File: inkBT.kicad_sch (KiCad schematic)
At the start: 10 parts, among them J1 AudioJack2_Ground, U1 LM2596S-3.3, U2 ESP32-WROOM-32, U3 PCM5102A

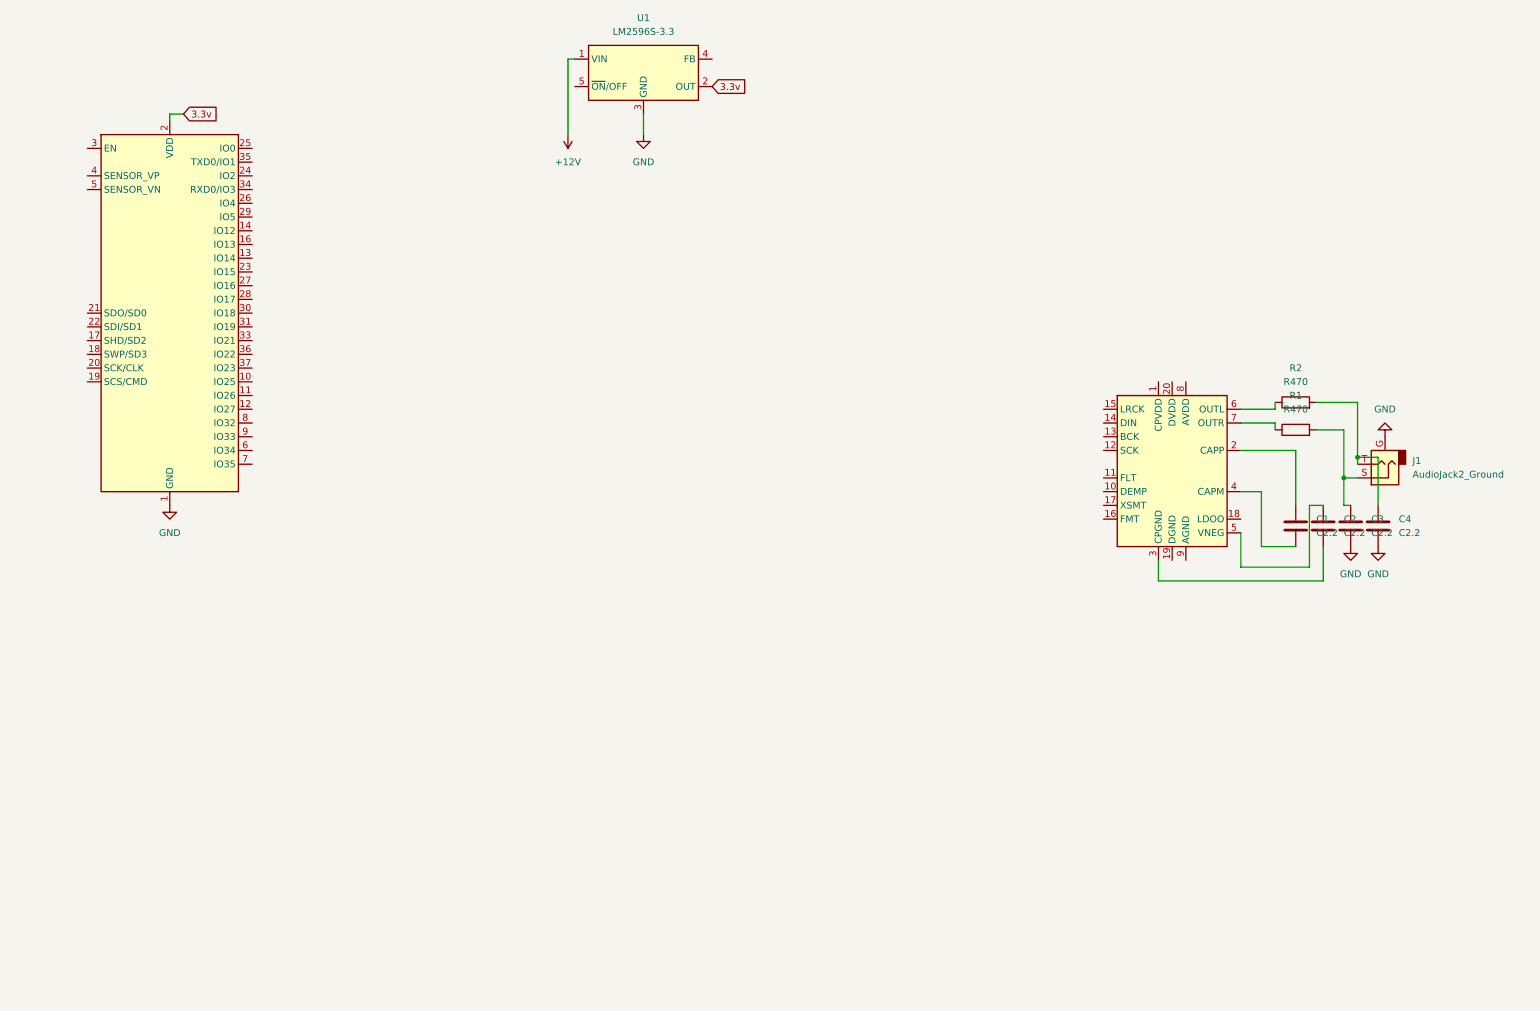
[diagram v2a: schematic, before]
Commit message: a
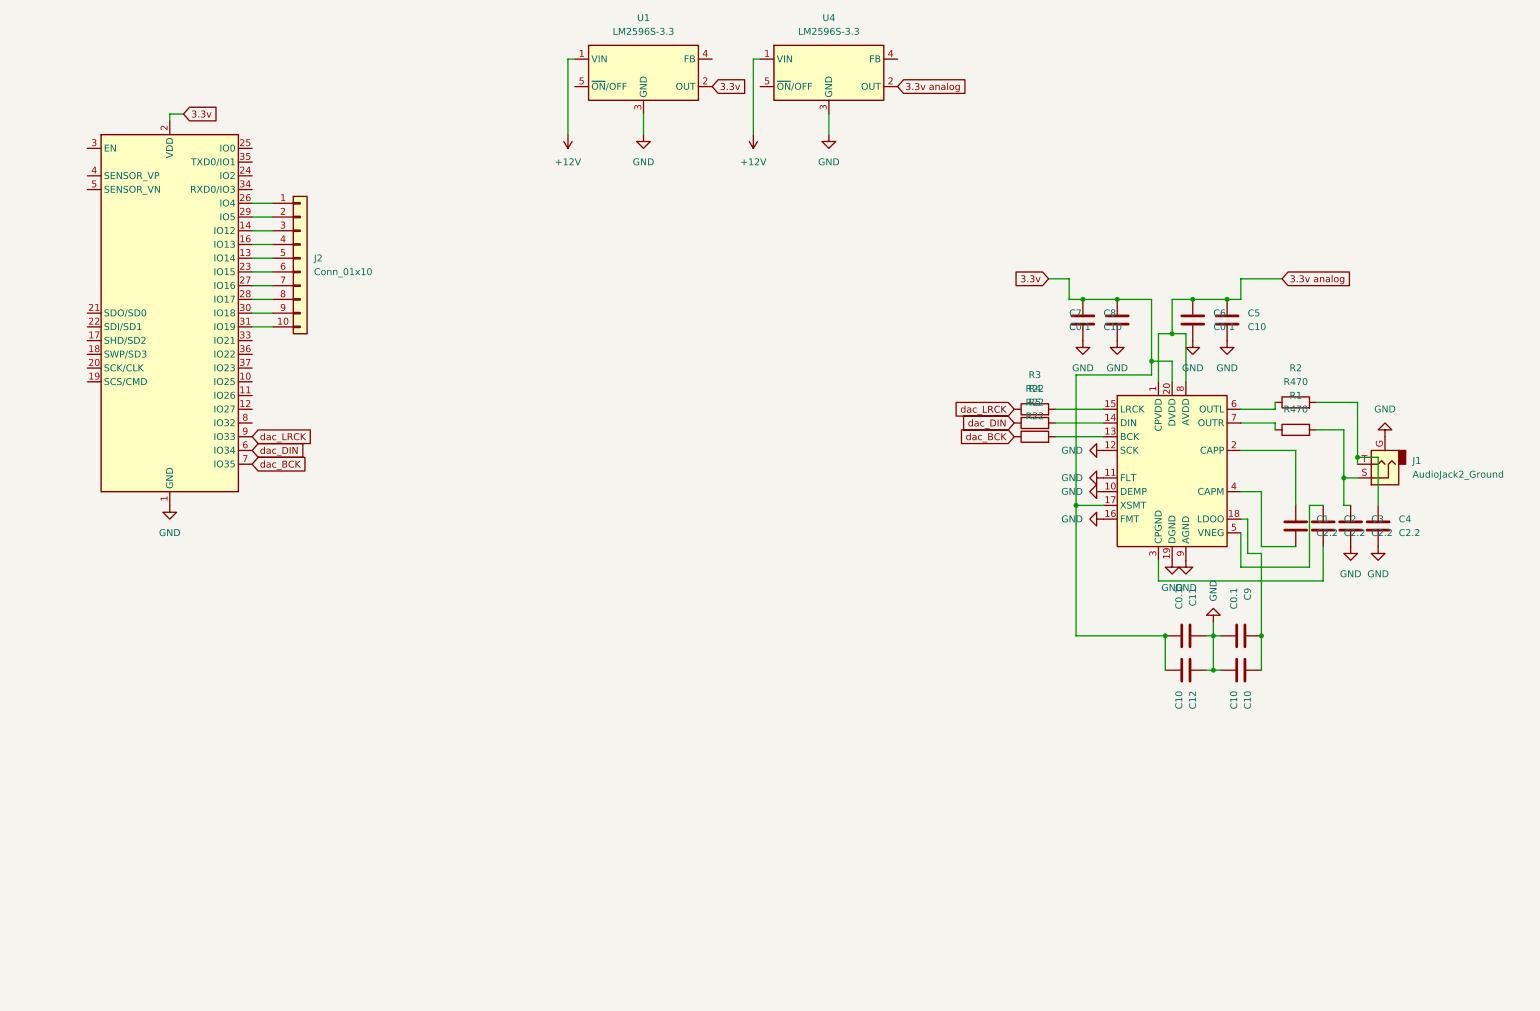
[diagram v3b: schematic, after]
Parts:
- added C10, C12, C5, C8: C10, Capacitor_SMD:C_1206_3216Metric_Pad1.33x1.80mm_HandSolder, symbol Device:C
- added C11, C6, C7, C9: C0.1, Capacitor_SMD:C_1206_3216Metric_Pad1.33x1.80mm_HandSolder, symbol Device:C
- added J2: Conn_01x10, symbol Connector_Generic:Conn_01x10
- added R3, R4, R5: R22, Resistor_SMD:R_1206_3216Metric_Pad1.30x1.75mm_HandSolder, symbol Device:R
- added U4: LM2596S-3.3, Package_TO_SOT_SMD:TO-263-5_TabPin3, symbol Regulator_Switching:LM2596S-3.3
- C1, C2, C3, C4: footprint Package_SO:SOIC-8_3.9x4.9mm_P1.27mm -> Capacitor_SMD:C_1206_3216Metric_Pad1.33x1.80mm_HandSolder
- J1: footprint Connector_Audio:Jack_3.5mm_QingPu_WQP-PJ398SM_Vertical_CircularHoles -> Connector_PinSocket_1.00mm:PinSocket_1x03_P1.00mm_Vertical
- R1, R2: footprint (none) -> Resistor_SMD:R_1206_3216Metric_Pad1.30x1.75mm_HandSolder
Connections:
- net +12V: now also U4.1 (VIN)
- net 3.3v: now also U3.17 (XSMT), U3.20 (DVDD), C11.2, C12.2, C7.1, C8.1
- net GND: now also U3.10 (DEMP), U3.11 (FLT), U3.12 (SCK), U3.16 (FMT), U3.19 (DGND), U3.9 (AGND), C10.2, C11.1, C12.1, C5.2, C6.2, C7.2, C8.2, C9.2, U4.3 (GND)
- net 3.3v analog: now reaches U3.1 (CPVDD)
- net 3.3v analog: now also U3.8 (AVDD), C5.1, C6.1, U4.2 (OUT)
- net at U3.13 (BCK): now also R5.2
- net at U3.14 (DIN): now also R4.2
- net at U3.15 (LRCK): now also R3.2
- net at U3.18 (LDOO): now also C10.1, C9.1
- net at U2.13 (IO14): now also J2.5 (Pin_5)
- net at U2.14 (IO12): now also J2.3 (Pin_3)
- net at U2.16 (IO13): now also J2.4 (Pin_4)
- net at U2.23 (IO15): now also J2.6 (Pin_6)
- net at U2.26 (IO4): now also J2.1 (Pin_1)
- net at U2.27 (IO16): now also J2.7 (Pin_7)
- net at U2.28 (IO17): now also J2.8 (Pin_8)
- net at U2.29 (IO5): now also J2.2 (Pin_2)
- net at U2.30 (IO18): now also J2.9 (Pin_9)
- net at U2.31 (IO19): now also J2.10 (Pin_10)
- net dac_DIN: now reaches U2.6 (IO34)
- net dac_DIN: now also R4.1
- net dac_BCK: now reaches U2.7 (IO35)
- net dac_BCK: now also R5.1
- net dac_LRCK: now reaches U2.9 (IO33)
- net dac_LRCK: now also R3.1

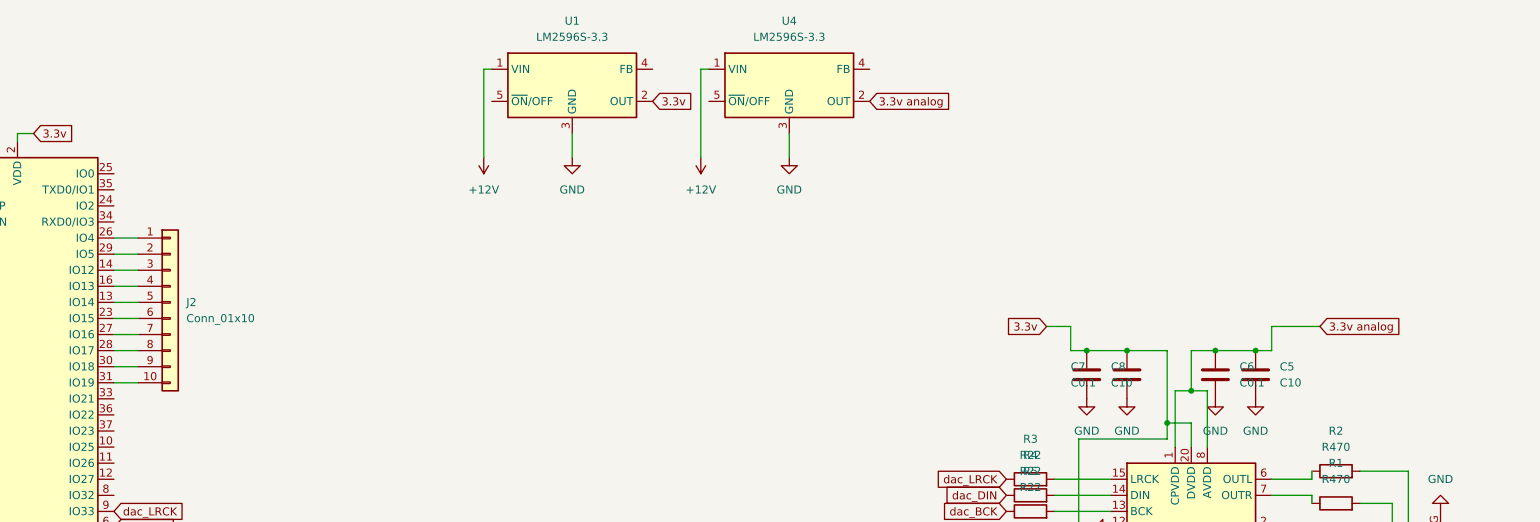
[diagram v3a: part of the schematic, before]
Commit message: a
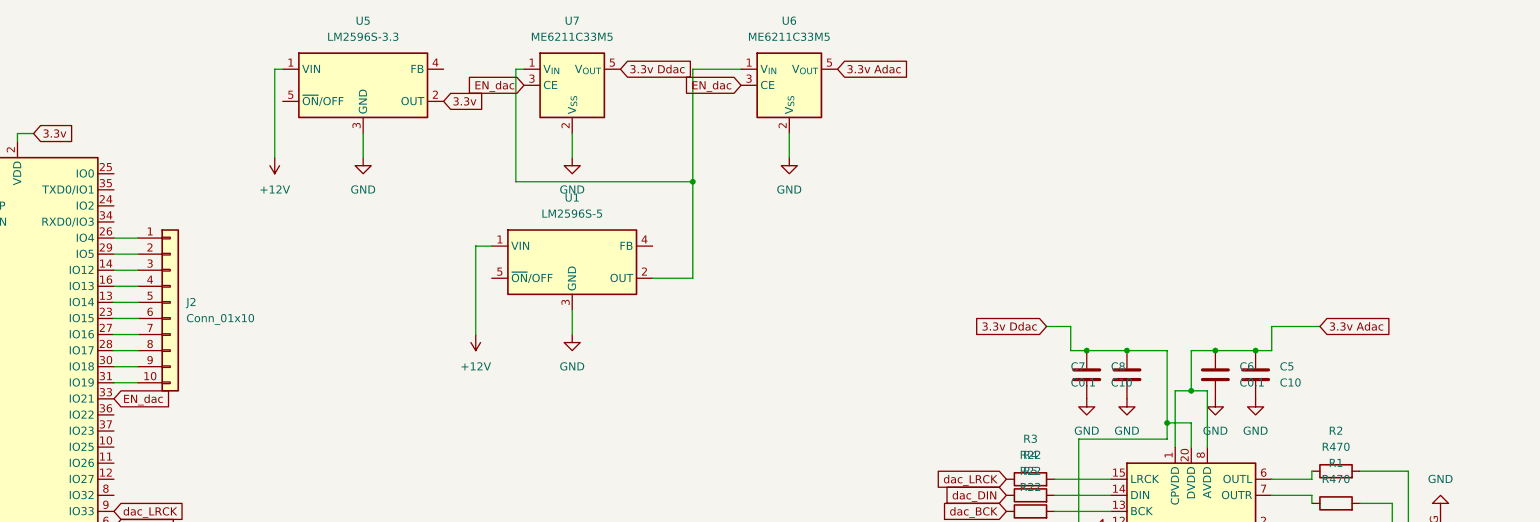
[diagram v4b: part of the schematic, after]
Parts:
- removed U1, U4: LM2596S-3.3, Package_TO_SOT_SMD:TO-263-5_TabPin3, symbol Regulator_Switching:LM2596S-3.3
- added U1: LM2596S-5, Package_TO_SOT_SMD:TO-263-5_TabPin3, symbol Regulator_Switching:LM2596S-5
- added U5: LM2596S-3.3, Package_TO_SOT_SMD:TO-263-5_TabPin3, symbol Regulator_Switching:LM2596S-3.3
- added U6, U7: ME6211C33M5, Package_TO_SOT_SMD:SOT-23-5, symbol Regulator_Linear:ME6211C33M5
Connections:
- net +12V: now also U1.1 (VIN), U5.1 (VIN)
- net 3.3v: now also U5.2 (OUT); no longer C11.2, C12.2, C7.1, C8.1, U3.17 (XSMT), U3.20 (DVDD)
- net GND: now also U1.3 (GND), U5.3 (GND), U6.2 (V_{SS}), U7.2 (V_{SS})
- net EN_dac: now reaches U2.33 (IO21)
- net EN_dac: now also U6.3 (CE), U7.3 (CE)
- net 3.3v analog renamed 3.3v Adac
- net 3.3v Adac: now also U6.5 (V_{OUT})
- new net: U1.2 (OUT), U6.1 (V_{IN}), U7.1 (V_{IN})
- new net 3.3v Ddac: C11.2, C12.2, C7.1, C8.1, U3.17 (XSMT), U3.20 (DVDD), U7.5 (V_{OUT})

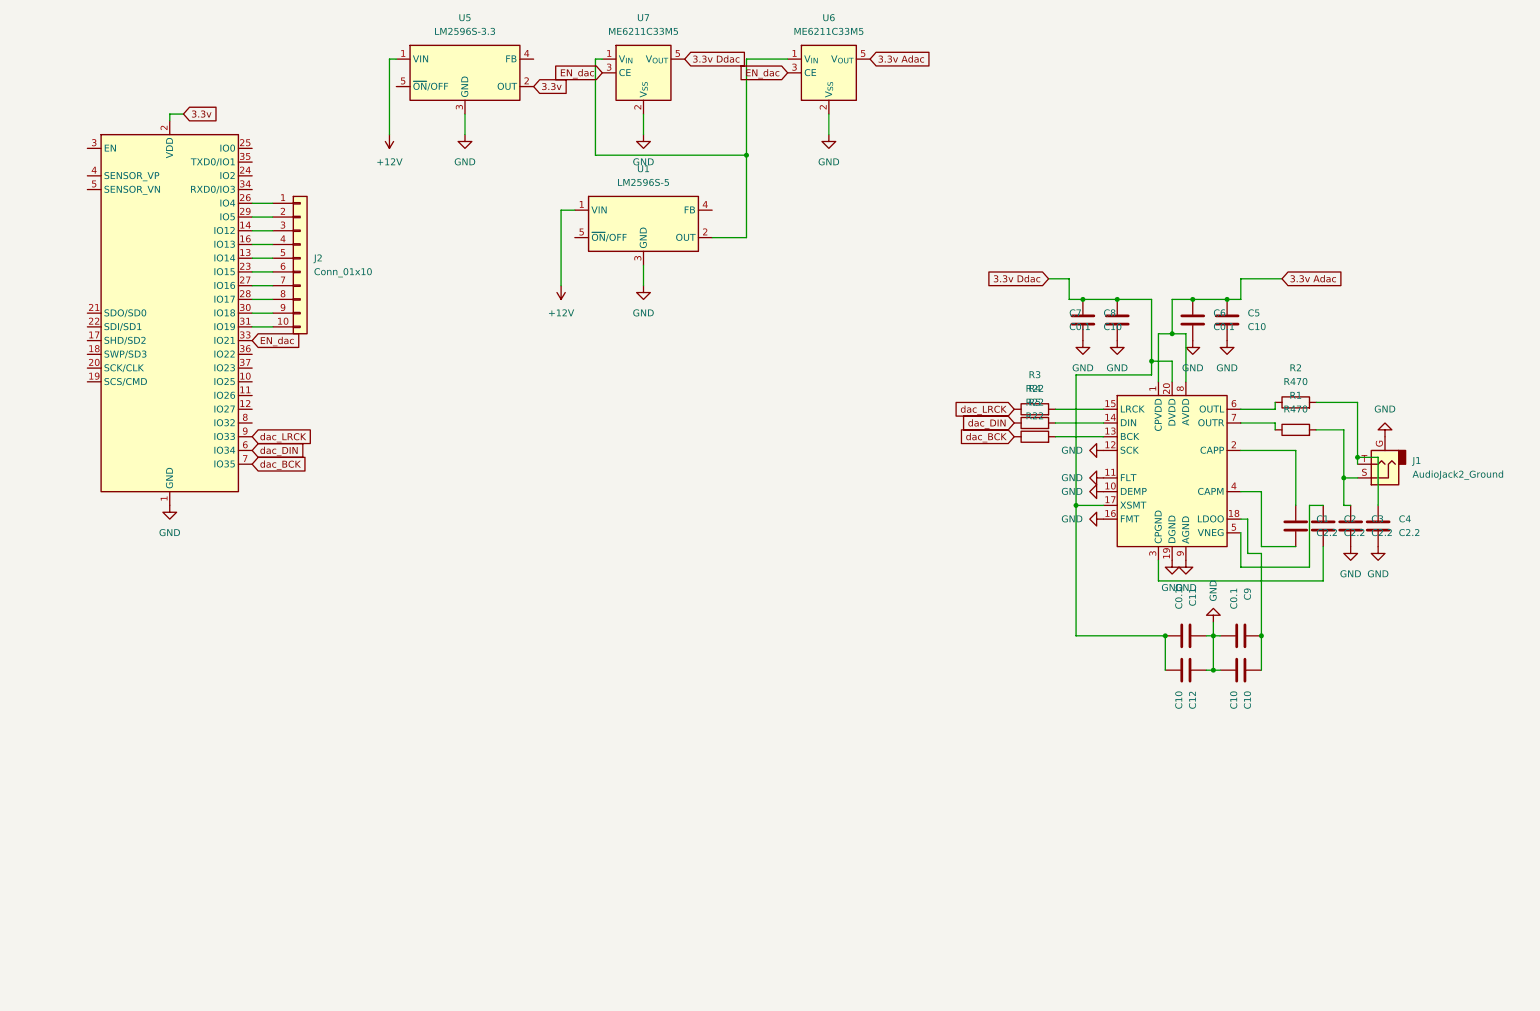
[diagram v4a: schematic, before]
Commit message: a
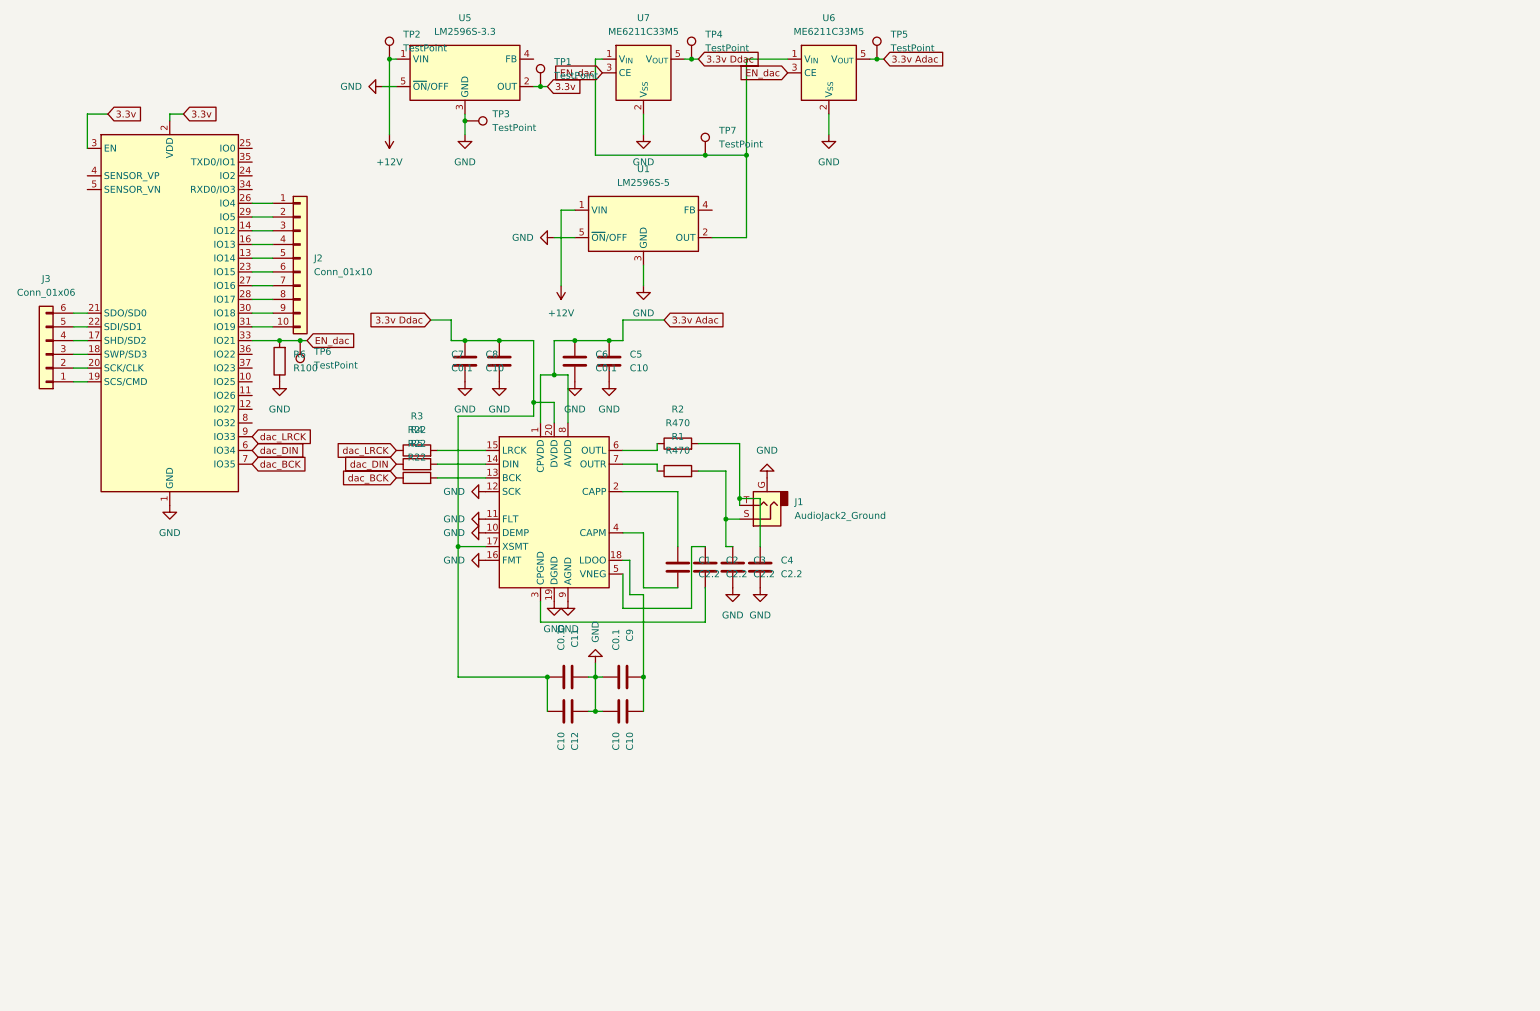
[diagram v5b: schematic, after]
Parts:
- added J3: Conn_01x06, Connector_PinHeader_2.00mm:PinHeader_1x06_P2.00mm_Vertical, symbol Connector_Generic:Conn_01x06
- added R6: R100, Resistor_SMD:R_1206_3216Metric_Pad1.30x1.75mm_HandSolder, symbol Device:R
- added TP1, TP2, TP3, TP4, TP5, TP6, TP7: TestPoint, TestPoint:TestPoint_Pad_D2.0mm, symbol Connector:TestPoint
- J2: footprint (none) -> Connector_PinHeader_2.00mm:PinHeader_1x10_P2.00mm_Vertical
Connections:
- net +12V: now also TP2.1
- net 3.3v: now also U2.3 (EN), TP1.1
- net 3.3v Adac: now also TP5.1
- net 3.3v Ddac: now also TP4.1
- net EN_dac: now also R6.2, TP6.1
- net GND: now also U1.5 (~{ON}/OFF), U5.5 (~{ON}/OFF), R6.1, TP3.1
- net at U1.2 (OUT), U6.1 (V_{IN}), U7.1 (V_{IN}): now also TP7.1
- net at U2.17 (SHD/SD2): now also J3.4 (Pin_4)
- net at U2.18 (SWP/SD3): now also J3.3 (Pin_3)
- net at U2.19 (SCS/CMD): now also J3.1 (Pin_1)
- net at U2.20 (SCK/CLK): now also J3.2 (Pin_2)
- net at U2.21 (SDO/SD0): now also J3.6 (Pin_6)
- net at U2.22 (SDI/SD1): now also J3.5 (Pin_5)
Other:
- moved on the sheet: C1, C10, C11, C12, C2, C3, C4, C5, C6, C7, C8, C9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
